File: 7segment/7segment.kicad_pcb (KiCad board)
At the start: 4 copper layers, 22.5 x 25.1 mm, 30 parts, among them J1 AVR-ISP-6, J2 Conn_01x10, J4 Conn_01x02, Q1 Q_NPN_BEC, Q2 Q_NPN_BEC, U1 ATmega168PA-AU, U2 HDSP-523

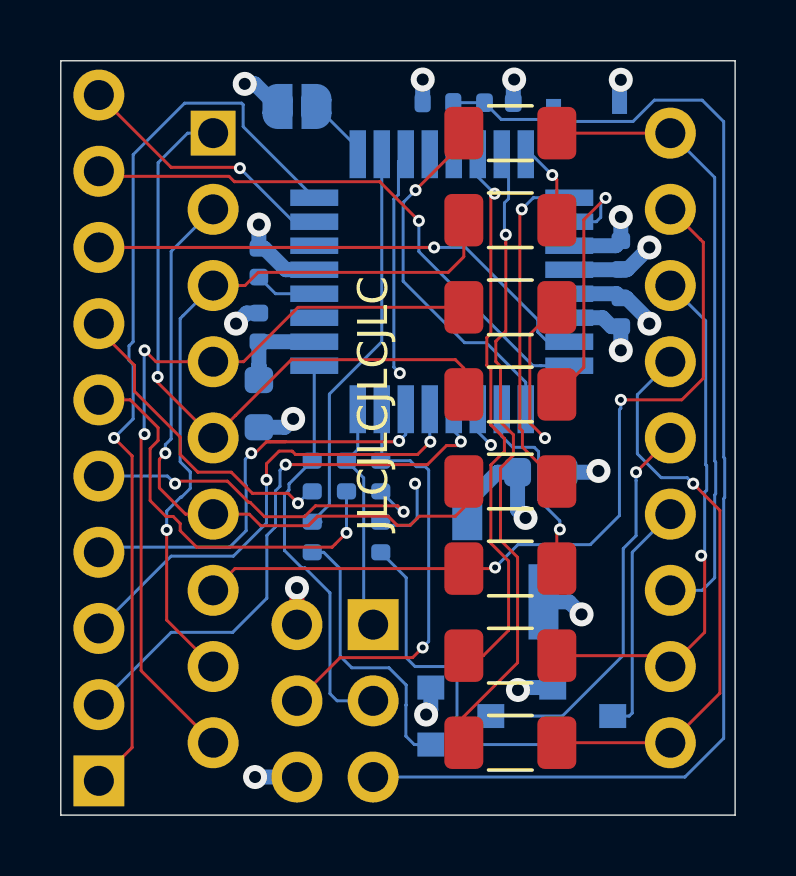
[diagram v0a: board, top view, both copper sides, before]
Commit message: Update 7 segment
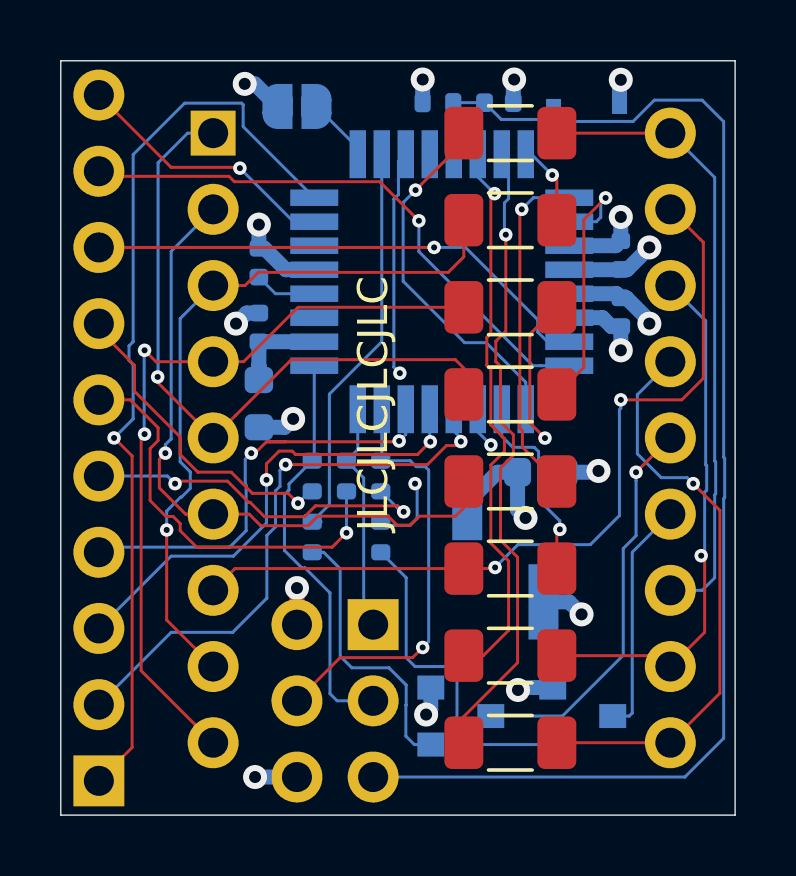
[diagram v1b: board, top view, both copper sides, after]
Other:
- net class Default: clearance 0.2 -> 0.127; trace_width 0.1 -> 0.127; via_dia 0.4 -> 0.45
- rule pad_to_mask_clearance: 0.0508 -> 0
- rule trace_clearance: 0.2 -> 0.127
- rule trace_min: 0.09 -> 0.1
- rule via_min_size: 0.4 -> 0.45
